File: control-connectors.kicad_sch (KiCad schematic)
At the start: 0 parts

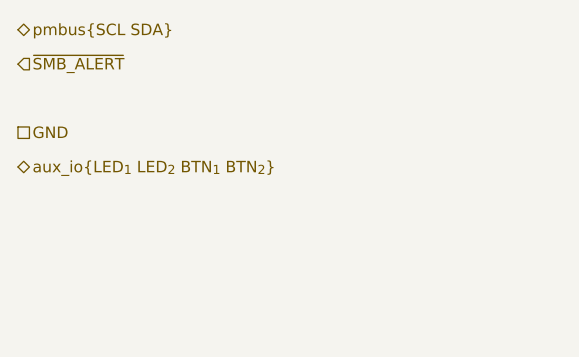
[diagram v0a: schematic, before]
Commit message: flesh out remote interface
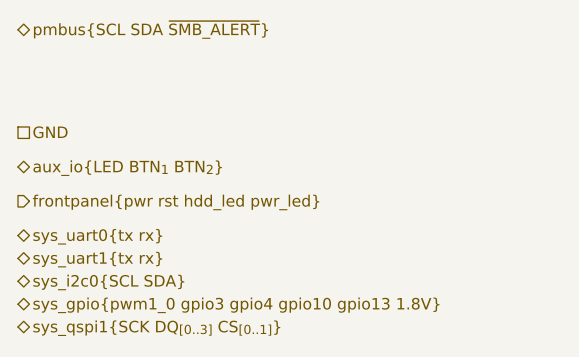
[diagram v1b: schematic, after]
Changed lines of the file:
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@@
     (rev "1")
   )
-  (hierarchical_label "pmbus{SCL SDA}" (shape bidirectional) (at 43.18 34.29 0)
-    (effects (font (size 1.27 1.27)) (justify left))
-  )
-  (hierarchical_label "~SMB_ALERT" (shape input) (at 43.18 38.1 0)
+  (hierarchical_label "pmbus{SCL SDA ~SMB_ALERT}" (shape bidirectional) (at 43.18 34.29 0)
     (effects (font (size 1.27 1.27)) (justify left))
   )
@@
     (effects (font (size 1.27 1.27)) (justify left))
   )
-  (hierarchical_label "aux_io{LED_{1} LED_{2} BTN_{1} BTN_{2}}" (shape bidirectional) (at 43.18 49.53 0)
+  (hierarchical_label "aux_io{LED BTN_{1} BTN_{2}}" (shape bidirectional) (at 43.18 49.53 0)
     (effects (font (size 1.27 1.27)) (justify left))
   )
+  (hierarchical_label "frontpanel{pwr rst hdd_led pwr_led}" (shape output) (at 43.18 53.34 0)
+    (effects (font (size 1.27 1.27)) (justify left))
+  )
+  (hierarchical_label "sys_uart0{tx rx}" (shape bidirectional) (at 43.18 57.15 0)
+    (effects (font (size 1.27 1.27)) (justify left))
+  )
+  (hierarchical_label "sys_uart1{tx rx}" (shape bidirectional) (at 43.18 59.69 0)
+    (effects (font (size 1.27 1.27)) (justify left))
+  )
+  (hierarchical_label "sys_i2c0{SCL SDA}" (shape bidirectional) (at 43.18 62.23 0)
+    (effects (font (size 1.27 1.27)) (justify left))
+  )
+  (hierarchical_label "sys_gpio{pwm1_0 gpio3 gpio4 gpio10 gpio13 1.8V}" (shape bidirectional) (at 43.18 64.77 0)
+    (effects (font (size 1.27 1.27)) (justify left))
+  )
+  (hierarchical_label "sys_qspi1{SCK DQ_{[0..3]} CS_{[0..1]}}" (shape bidirectional) (at 43.18 67.31 0)
+    (effects (font (size 1.27 1.27)) (justify left))
+  )
